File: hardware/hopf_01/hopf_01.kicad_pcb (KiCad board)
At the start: 2 copper layers, 120.2 x 120.2 mm, 257 parts, among them J1 SMA_50R, J2 SMA_50R, J3 SMA_50R, J4 SMA_50R

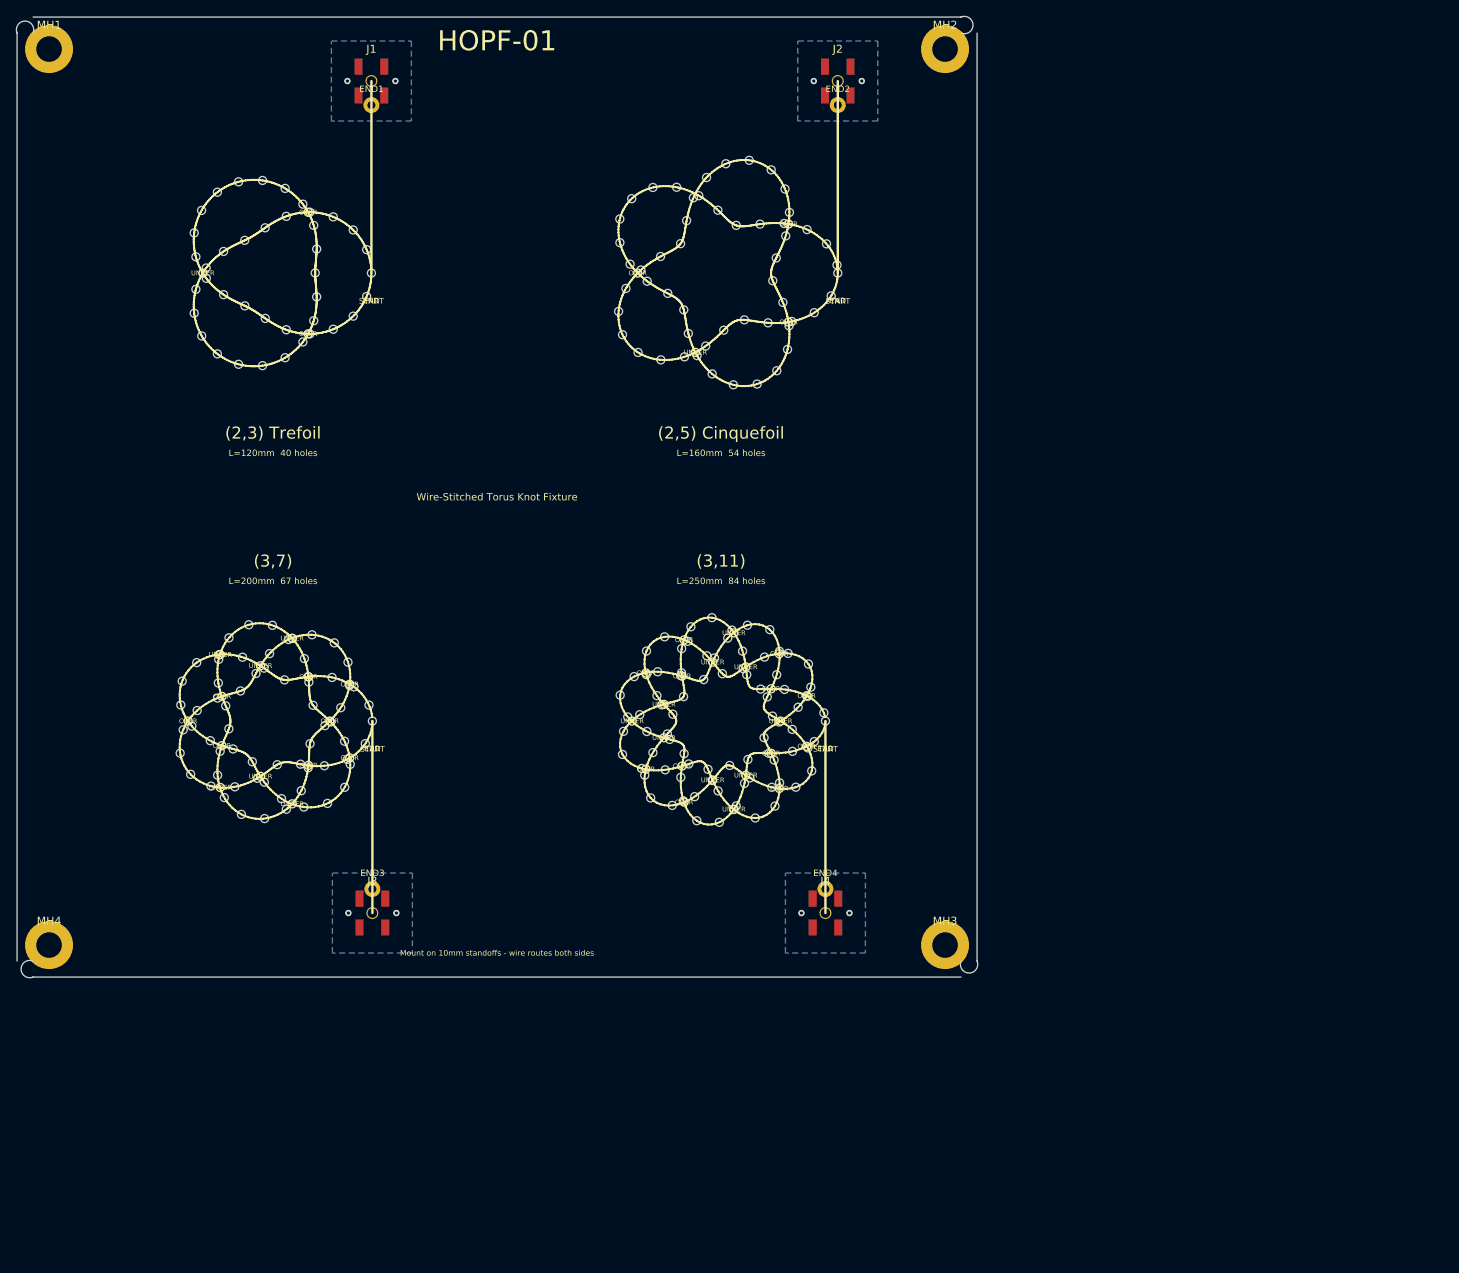
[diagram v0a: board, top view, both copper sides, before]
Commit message: updated table
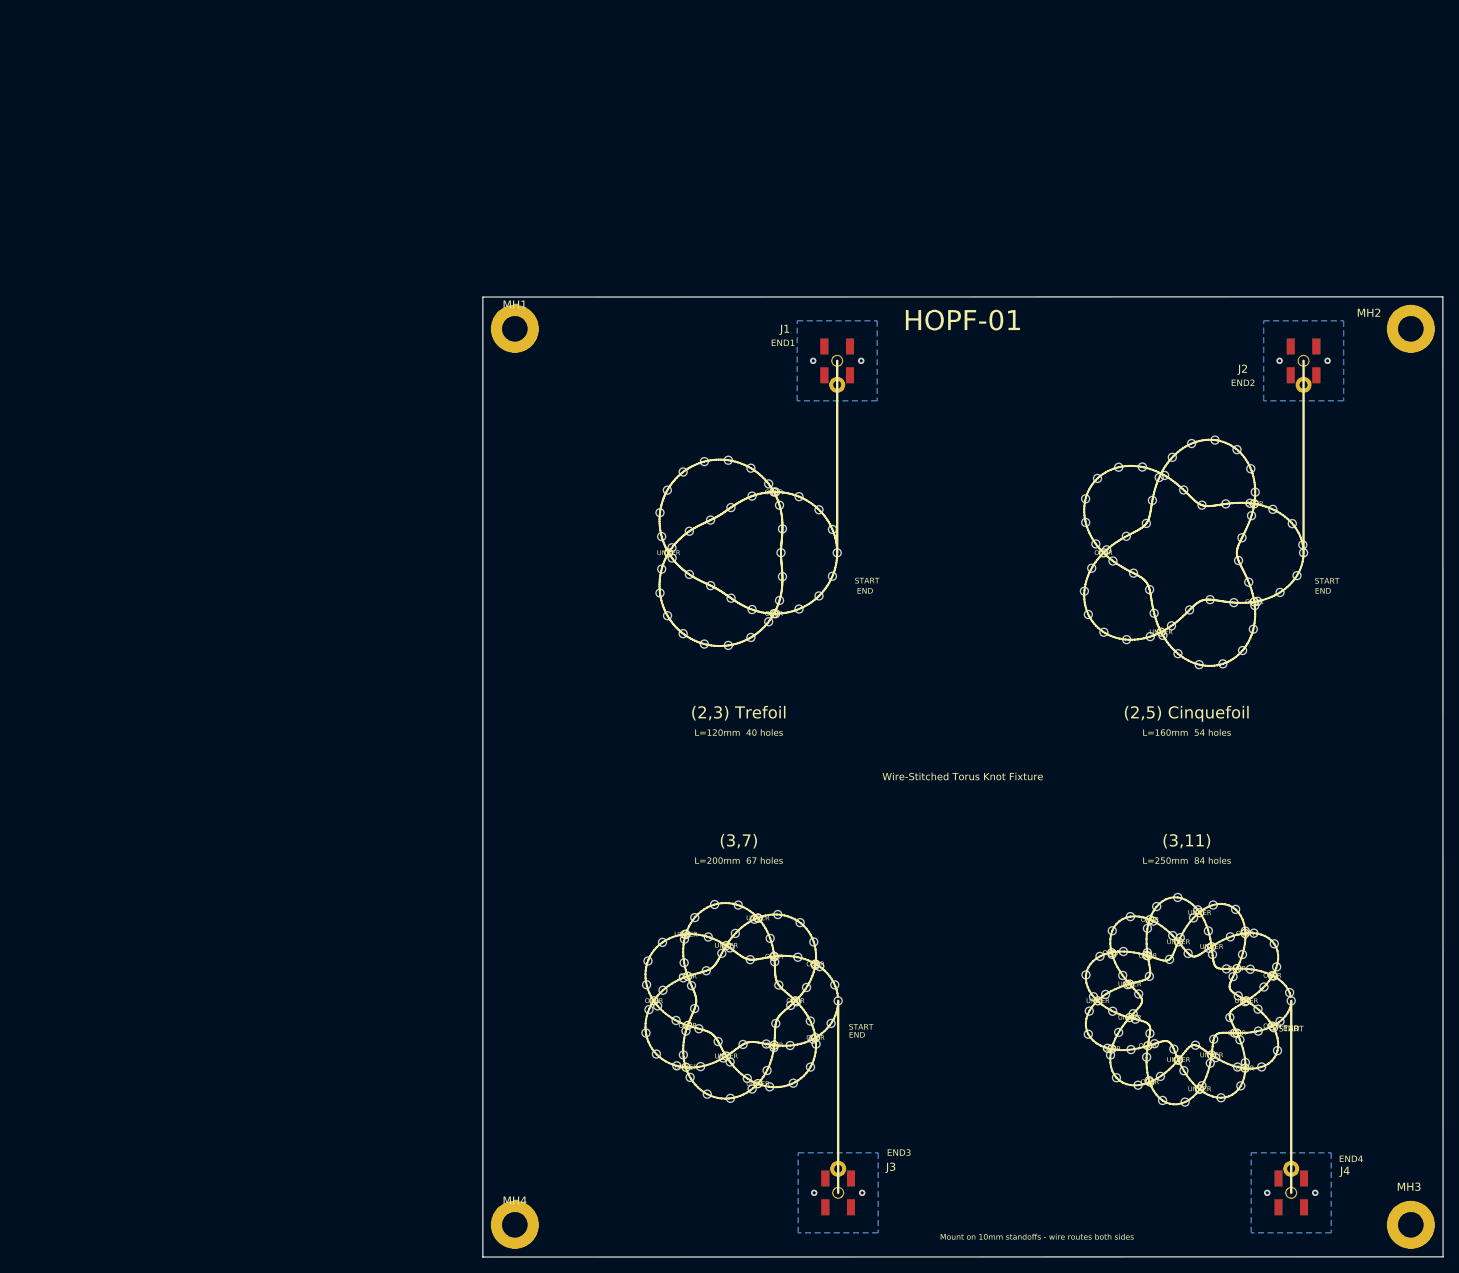
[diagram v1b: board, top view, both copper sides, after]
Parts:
- moved ? 67.9 mm to (139.6, 69.5)
- moved ? 67.9 mm to (88.1, 117.0)
- moved ? 67.9 mm to (94.6, 128.8)
- moved ? 67.9 mm to (146.6, 74.1)
- moved ? 67.9 mm to (86.7, 62.9)
- moved ? 67.9 mm to (91.7, 56.4)
- moved ? 67.9 mm to (80.4, 72.0)
- moved ? 67.9 mm to (136.9, 117.2)
- moved ? 67.9 mm to (154.2, 56.5)
- moved ? 67.9 mm to (81.3, 74.8)
- moved ? 67.9 mm to (88.9, 55.4)
- moved ? 67.9 mm to (80.4, 61.9)
- moved ? 67.9 mm to (148.9, 114.2)
- moved ? 67.9 mm to (157.9, 125.5)
- moved ? 67.9 mm to (84.7, 123.9)
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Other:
- board size 120.2 x 120.2 mm -> 120 x 120 mm
